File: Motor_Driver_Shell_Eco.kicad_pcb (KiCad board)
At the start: 6 copper layers, 119.6 x 167.9 mm, 214 parts, among them J1 I2C EKRAN, J11 USB_C_Receptacle, J12 Conn_01x02, J13 OUTSIDE LED, J2 HALL INPUT, J3 Conn_01x02, J4 Conn_01x02, J5 Conn_01x04, J6 Conn_01x06, J7 Conn_01x02, J8 Conn_01x03, J9 Conn_01x03, Q1 BC817, Q14 IAUS300N08S5N0, Q15 IAUS300N08S5N0, Q16 IAUS300N08S5N0, Q17 IAUS300N08S5N0, Q18 IAUS300N08S5N0, Q19 IAUS300N08S5N0, Q2 BC817, Q20 IAUS300N08S5N0, Q21 IAUS300N08S5N0, Q6 IAUS300N08S5N0, Q7 IAUS300N08S5N0, Q8 IAUS300N08S5N0, Q9 IAUS300N08S5N0, SW1 SW_Push, SW2 SW_Push, U1 STM32G474VETx, U10 IRS21867S, U11 INA241A2, U12 TMP101, U13 INA241A2, U2 LM5017MR, U3 AP2204K-5.0, U4 XC6206 - 3V3, U5 INA241A2, U6 IRS21867S, U8 TJA1051T, U9 IRS21867S, Y1 8MHz

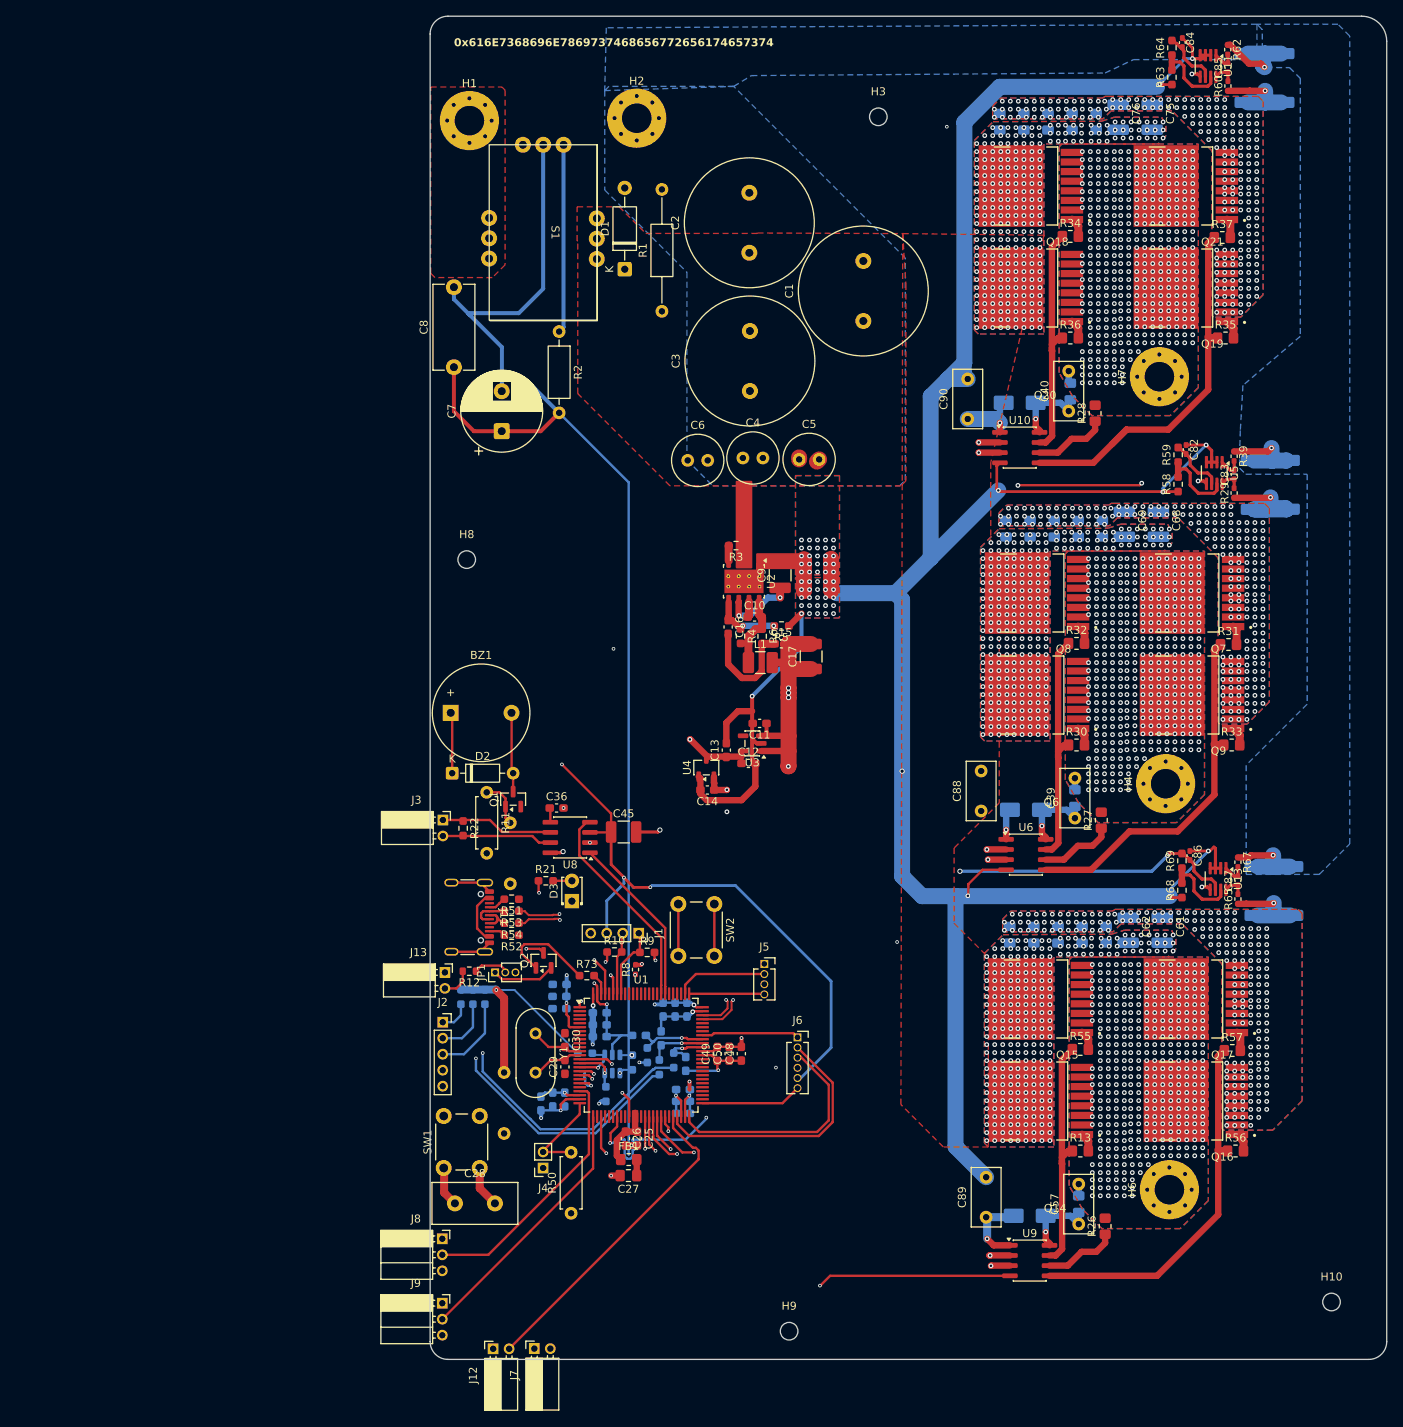
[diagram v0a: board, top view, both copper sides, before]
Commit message: rev3
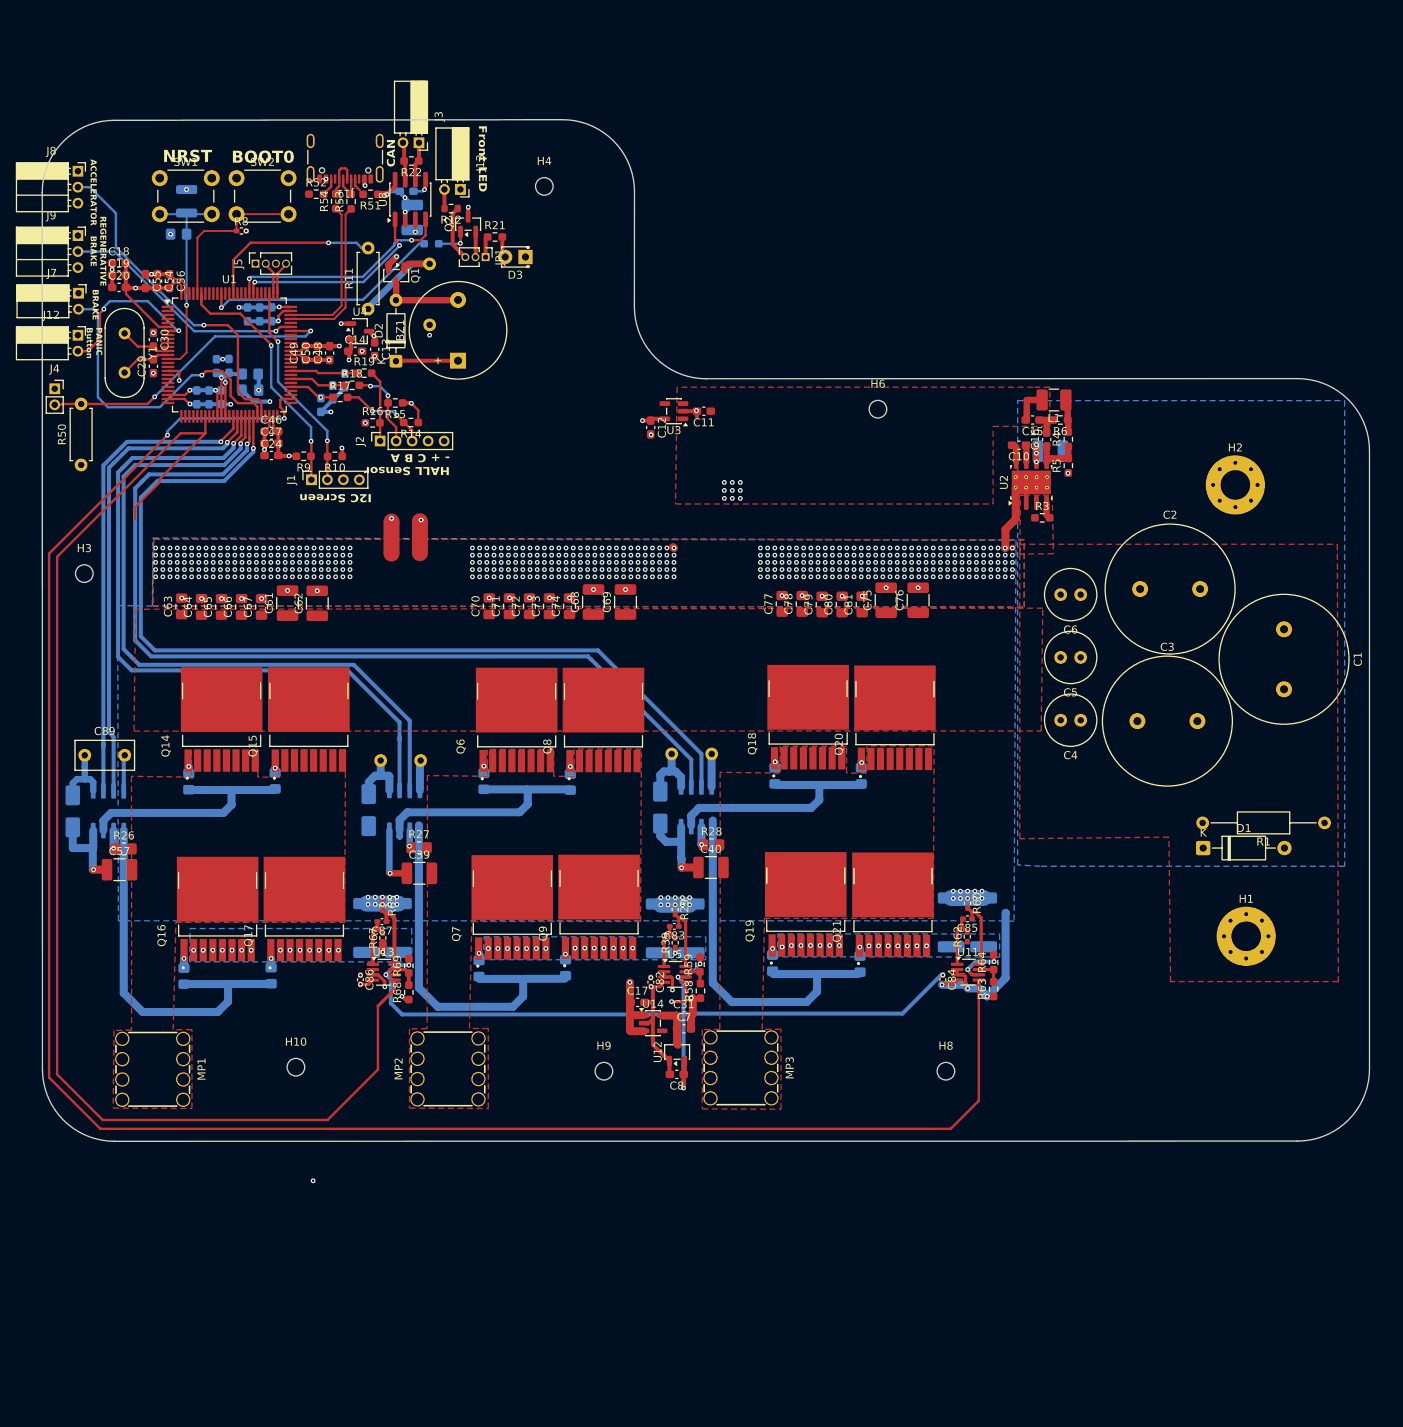
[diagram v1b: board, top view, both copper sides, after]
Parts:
- removed C58, C59, C60: 100uf, Capacitor_SMD:C_0805_2012Metric_Pad1.18x1.45mm_HandSolder
- removed H7: PHASE_C, MountingHole:MountingHole_3.7mm_Pad_Via
- removed J6: Conn_01x06, Connector_PinSocket_1.27mm:PinSocket_1x06_P1.27mm_Vertical
- removed R2: 1K, Resistor_THT:R_Axial_DIN0207_L6.3mm_D2.5mm_P10.16mm_Horizontal
- removed R23: 100, Resistor_SMD:R_0603_1608Metric_Pad0.98x0.95mm_HandSolder
- removed R24, R25: 4.7K, Resistor_SMD:R_0603_1608Metric_Pad0.98x0.95mm_HandSolder
- removed S1: LES50-NP, LES-50NP:LES50NP
- added C31: 2.2uF, Capacitor_SMD:C_0603_1608Metric_Pad1.08x0.95mm_HandSolder, F.Cu at (121.7, 144.6)
- added G***: LOGO, LOGO, B.Cu at (173.7, 134.1)
- added MP1: Phase_A, WP-BUTR:WP-BUTR_7460307, F.Cu at (55.4, 151.3)
- added MP2: Phase_B, WP-BUTR:WP-BUTR_7460307, F.Cu at (92.3, 151.2)
- added MP3: Phase_A, WP-BUTR:WP-BUTR_7460307, F.Cu at (128.9, 151.1)
- added U14: AP2204K-5.0, Package_TO_SOT_SMD:SOT-23-5, F.Cu at (117.9, 145.5)
- C17: value 47uF -> 1uF; footprint Capacitor_SMD:C_1210_3225Metric_Pad1.33x2.70mm_HandSolder -> Capacitor_SMD:C_0603_1608Metric_Pad1.08x0.95mm_HandSolder
- C18, C19, C20, C24, C46, C47, C54, C55, C56, C61, C62, C63, C64, C65, C66, C67, C68, C69, C70, C71, C72, C73, C74, C75, C76, C77, C78, C79, C80, C81, NT2, NT7, R14, R15, R16, R17, R18, R19: moved to F.Cu
- C25, C26, C27, C36, C45, C88, C9, C90, FB1, R13, R30, R31, R32, R33, R34, R35, R36, R37, R55, R56, R57, R73, U10, U6, U9: moved to B.Cu
- C28: footprint Capacitor_THT:C_Disc_D10.5mm_W5.0mm_P5.00mm -> Resistor_SMD:R_0805_2012Metric_Pad1.20x1.40mm_HandSolder; moved to B.Cu
- C39, C40, C57: footprint Capacitor_THT:C_Rect_L7.2mm_W3.5mm_P5.00mm_FKS2_FKP2_MKS2_MKP2 -> Capacitor_SMD:C_1210_3225Metric_Pad1.33x2.70mm_HandSolder
- C7: value 470uF/25V -> 1uF; footprint Capacitor_THT:CP_Radial_D10.0mm_P5.00mm -> Capacitor_SMD:C_0603_1608Metric_Pad1.08x0.95mm_HandSolder
- C8: value 100nF -> 2.2uF; footprint Capacitor_THT:C_Disc_D10.5mm_W5.0mm_P10.00mm -> Capacitor_SMD:C_0603_1608Metric_Pad1.08x0.95mm_HandSolder
- H4: value PHASE_B -> MountingHole; footprint MountingHole:MountingHole_3.7mm_Pad_Via -> MountingHole:MountingHole_2.2mm_M2
- H6: value PHASE_A -> MountingHole; footprint MountingHole:MountingHole_3.7mm_Pad_Via -> MountingHole:MountingHole_2.2mm_M2
- R7: footprint Resistor_THT:R_Axial_DIN0207_L6.3mm_D2.5mm_P7.62mm_Horizontal -> Resistor_SMD:R_1210_3225Metric
- U12: value TMP101 -> XC6206 - 3V3; footprint Package_TO_SOT_SMD:SOT-23-6 -> Package_TO_SOT_SMD:SOT-23-3; moved to F.Cu
- moved J7 143.7 mm to (46.1, 54.2), turned to 0 degrees
- moved J8 141.0 mm to (46.0, 39.0)
- moved J9 141.0 mm to (46.0, 47.0)
- moved H1 140.8 mm to (192.0, 134.6)
- moved J12 136.9 mm to (46.0, 59.5), turned to 0 degrees
- moved R56 133.2 mm to (59.3, 139.6), turned to 90 degrees
- moved H10 132.7 mm to (73.2, 151.0)
- moved R26 131.4 mm to (51.8, 123.7), turned to 0 degrees
- moved D7 129.9 mm to (45.4, 119.0), turned to 90 degrees
- moved SW1 128.7 mm to (56.2, 39.9), turned to 0 degrees
- moved U9 128.1 mm to (49.8, 118.9), turned to -90 degrees
- moved C57 127.8 mm to (51.2, 126.3), turned to 0 degrees
- moved C89 126.6 mm to (46.9, 112.0), turned to 0 degrees
- moved C28 126.0 mm to (58.6, 46.9)
- moved Q16 124.7 mm to (63.5, 131.4), turned to 90 degrees
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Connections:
- C11 pad 2: GND -> -VDC
- C12 pad 2: GND -> -VDC
- C17 pad 2: +12V -> -VDC
- C7 pad 1: CSense_OUT_LES -> +5VD
- C7 pad 2: GND -> -VDC
- C8 pad 1: CSense_OUT_LES -> +3V3F
- C8 pad 2: GND -> -VDC
- C82 pad 1: +3V3 -> +3V3F
- C82 pad 2: GND -> -VDC
- C84 pad 1: +3V3 -> +3V3F
- C84 pad 2: GND -> -VDC
- C86 pad 1: +3V3 -> +3V3F
- C86 pad 2: GND -> -VDC
- C88 pad 2: GND -> -VDC
- C89 pad 2: GND -> -VDC
- C90 pad 2: GND -> -VDC
- H1 pad 1: Net-(H1-Pad1) -> +VDC
- Q16 pad 2: -VDC -> Net-(Q16-Pad2)
- Q16 pad 3: -VDC -> Net-(Q16-Pad2)
- Q16 pad 4: -VDC -> Net-(Q16-Pad2)
- Q16 pad 5: -VDC -> Net-(Q16-Pad2)
- Q16 pad 6: -VDC -> Net-(Q16-Pad2)
- Q16 pad 7: -VDC -> Net-(Q16-Pad2)
- Q16 pad 8: -VDC -> Net-(Q16-Pad2)
- Q17 pad 2: -VDC -> Net-(Q16-Pad2)
- Q17 pad 3: -VDC -> Net-(Q16-Pad2)
- Q17 pad 4: -VDC -> Net-(Q16-Pad2)
- Q17 pad 5: -VDC -> Net-(Q16-Pad2)
- Q17 pad 6: -VDC -> Net-(Q16-Pad2)
- Q17 pad 7: -VDC -> Net-(Q16-Pad2)
- Q17 pad 8: -VDC -> Net-(Q16-Pad2)
- Q19 pad 2: -VDC -> Net-(Q19-Pad2)
- Q19 pad 3: -VDC -> Net-(Q19-Pad2)
- Q19 pad 4: -VDC -> Net-(Q19-Pad2)
- Q19 pad 5: -VDC -> Net-(Q19-Pad2)
- Q19 pad 6: -VDC -> Net-(Q19-Pad2)
- Q19 pad 7: -VDC -> Net-(Q19-Pad2)
- Q19 pad 8: -VDC -> Net-(Q19-Pad2)
- Q2 pad 2: Net-(JP1-A) -> Net-(JP1-C)
- Q21 pad 2: -VDC -> Net-(Q19-Pad2)
- Q21 pad 3: -VDC -> Net-(Q19-Pad2)
- Q21 pad 4: -VDC -> Net-(Q19-Pad2)
- Q21 pad 5: -VDC -> Net-(Q19-Pad2)
- Q21 pad 6: -VDC -> Net-(Q19-Pad2)
- Q21 pad 7: -VDC -> Net-(Q19-Pad2)
- Q21 pad 8: -VDC -> Net-(Q19-Pad2)
- Q7 pad 2: -VDC -> Net-(Q7-Pad2)
- Q7 pad 3: -VDC -> Net-(Q7-Pad2)
- Q7 pad 4: -VDC -> Net-(Q7-Pad2)
- Q7 pad 5: -VDC -> Net-(Q7-Pad2)
- Q7 pad 6: -VDC -> Net-(Q7-Pad2)
- Q7 pad 7: -VDC -> Net-(Q7-Pad2)
- Q7 pad 8: -VDC -> Net-(Q7-Pad2)
- Q9 pad 2: -VDC -> Net-(Q7-Pad2)
- Q9 pad 3: -VDC -> Net-(Q7-Pad2)
- Q9 pad 4: -VDC -> Net-(Q7-Pad2)
- Q9 pad 5: -VDC -> Net-(Q7-Pad2)
- Q9 pad 6: -VDC -> Net-(Q7-Pad2)
- Q9 pad 7: -VDC -> Net-(Q7-Pad2)
- Q9 pad 8: -VDC -> Net-(Q7-Pad2)
- R12 pad 1: Net-(JP1-C) -> Net-(JP1-B)
- R21 pad 1: Net-(JP1-B) -> Net-(JP1-A)
- R38 pad 2: -VDC -> Net-(Q7-Pad2)
- R39 pad 1: -VDC -> Net-(Q7-Pad2)
- R5 pad 1: GND -> -VDC
- R58 pad 1: GND -> -VDC
- R59 pad 2: +3V3 -> +3V3F
- R61 pad 2: -VDC -> Net-(Q19-Pad2)
- R62 pad 1: -VDC -> Net-(Q19-Pad2)
- R63 pad 1: GND -> -VDC
- R64 pad 2: +3V3 -> +3V3F
- R66 pad 1: -VDC -> Net-(Q16-Pad2)
- R67 pad 1: -VDC -> Net-(Q16-Pad2)
- R68 pad 1: GND -> -VDC
- R69 pad 2: +3V3 -> +3V3F
- R70 pad 2: -VDC -> Net-(Q7-Pad2)
- R71 pad 2: -VDC -> Net-(Q16-Pad2)
- R72 pad 2: -VDC -> Net-(Q19-Pad2)
- U1 pad 1: BRAKE -> unconnected-(U1-PE2-Pad1)
- U1 pad 15: TMP_SDA -> unconnected-(U1-PC0-Pad15)
- U1 pad 16: TMP_SCL -> unconnected-(U1-PC1-Pad16)
- U1 pad 18: TMP_ALERT -> unconnected-(U1-PC3-Pad18)
- U1 pad 20: CSense_OUT_LES -> unconnected-(U1-PA0-Pad20)
- U1 pad 21: B_VOL_CHECK -> unconnected-(U1-PA1-Pad21)
- U1 pad 22: ACCEL -> unconnected-(U1-PA2-Pad22)
- U1 pad 25: TEMP_SENSOR -> unconnected-(U1-PA3-Pad25)
- U1 pad 26: REGEN -> unconnected-(U1-PA4-Pad26)
- U1 pad 28: Current Sense_A -> unconnected-(U1-PA6-Pad28)
- U1 pad 32: Current_Sense_C -> Current Sense_A
- U1 pad 39: /FET/LS_MOS_A -> /FET/HS_MOS_A
- U1 pad 40: /FET/HS_MOS_A -> /FET/LS_MOS_A
- U1 pad 45: unconnected-(U1-PE14-Pad45) -> BRAKE
- U1 pad 46: PANIC STOP -> ACCEL
- U1 pad 47: BT_TX -> unconnected-(U1-PB10-Pad47)
- U1 pad 50: BT_RX -> unconnected-(U1-PB11-Pad50)
- U1 pad 51: BT_KEY -> unconnected-(U1-PB12-Pad51)
- U1 pad 52: unconnected-(U1-PB13-Pad52) -> Current_Sense_C
- U1 pad 55: unconnected-(U1-PD8-Pad55) -> HALL_C
- U1 pad 57: unconnected-(U1-PD10-Pad57) -> HALL_B
- U1 pad 59: unconnected-(U1-PD12-Pad59) -> HALL_A
- U1 pad 65: HALL_A -> unconnected-(U1-PC6-Pad65)
- U1 pad 66: HALL_B -> unconnected-(U1-PC7-Pad66)
- U1 pad 67: HALL_C -> unconnected-(U1-PC8-Pad67)
- U1 pad 68: BT_STATE -> unconnected-(U1-PC9-Pad68)
- U1 pad 69: unconnected-(U1-PA8-Pad69) -> TEMP_SENSOR
- U1 pad 7: unconnected-(U1-PC13-Pad7) -> PANIC STOP
- U1 pad 70: unconnected-(U1-PA9-Pad70) -> REGEN
- U1 pad 78: unconnected-(U1-PA15-Pad78) -> /MCU/I2C_SDA
- U1 pad 87: unconnected-(U1-PD5-Pad87) -> BUZZER
- U1 pad 90: unconnected-(U1-PB3-Pad90) -> STATUS_LED
- U1 pad 93: /MCU/I2C_SCL -> unconnected-(U1-PB6-Pad93)
- U1 pad 94: /MCU/I2C_SDA -> unconnected-(U1-PB7-Pad94)
- U1 pad 95: /MCU/BOOT0 -> /MCU/I2C_SCL
- U1 pad 96: unconnected-(U1-PB9-Pad96) -> /MCU/BOOT0
- U1 pad 97: BUZZER -> unconnected-(U1-PE0-Pad97)
- U1 pad 98: STATUS_LED -> unconnected-(U1-PE1-Pad98)
- U10 pad 4: GND -> -VDC
- U11 pad 2: GND -> -VDC
- U11 pad 3: GND -> -VDC
- U11 pad 4: GND -> -VDC
- U11 pad 6: +3V3 -> +3V3F
- U12 pad 1: TMP_SCL -> -VDC
- U12 pad 2: GND -> +3V3F
- U12 pad 3: TMP_ALERT -> +5VD
- U13 pad 2: GND -> -VDC
- U13 pad 3: GND -> -VDC
- U13 pad 4: GND -> -VDC
- U13 pad 6: +3V3 -> +3V3F
- U3 pad 2: GND -> -VDC
- U5 pad 2: GND -> -VDC
- U5 pad 3: GND -> -VDC
- U5 pad 4: GND -> -VDC
- U5 pad 6: +3V3 -> +3V3F
- U6 pad 4: GND -> -VDC
- U9 pad 4: GND -> unconnected-(U9-COM-Pad4)
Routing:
- net GND: track 585.4 -> 60.9 mm, vias 52 -> 24
- net +5V: track 258.3 -> 23.7 mm, vias 5 -> 6
- net +3V3: track 141.4 -> 10.6 mm, vias 15 -> 11
- net CSense_OUT_LES: track 125.4 -> 0.00 mm, vias 1 -> 0
- net +3V3F: track 0.00 -> 121.2 mm, vias 0 -> 10
- net -VDC: track 76.8 -> 154.9 mm, vias 673 -> 528
- net Current Sense_A: track 103.0 -> 163.3 mm, vias 3 -> 0
- net Current_Sense_C: track 200.7 -> 241.5 mm, vias 4 -> 2
- net Net-(J2-Pin_1): track 44.9 -> 8.93 mm, vias 1 -> 0
- net Net-(J2-Pin_3): track 46.2 -> 11.2 mm, vias 1 -> 2
- net Net-(J2-Pin_2): track 43.9 -> 10.3 mm, vias 1 -> 2
- net BT_TX: track 32.8 -> 0.00 mm
- net Current Sense_B: track 163.4 -> 192.8 mm, vias 4 -> 2
- net BT_RX: track 29.1 -> 0.00 mm
- net STATUS_LED: track 2.64 -> 30.4 mm, vias 0 -> 1
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- added copper zone on F.Cu, net +12V
- added copper zone on In2.Cu, net +3V3
- added copper zone on In2.Cu, net +5V
- added copper zone on B.Cu, net Net-(Q16-Pad2)
- added copper zone on B.Cu, net Net-(Q19-Pad2)
- added copper zone on B.Cu, net Net-(Q7-Pad2)
- removed copper zone on In3.Cu, net +3V3
- removed copper zone on B.Cu, net +VDC
- removed copper zone on In1.Cu, net +VDC
- removed copper zone on In2.Cu, net +VDC
- removed copper zone on In4.Cu, net +VDC
- removed copper zone on In1.Cu, net -VDC
- removed copper zone on In3.Cu, net -VDC
- removed copper zone on In4.Cu, net -VDC
- removed copper zone on B.Cu, net /FET/Phase_A_FET/PHASE_A
- removed copper zone on In2.Cu, net /FET/Phase_A_FET/PHASE_A
- removed copper zone on In3.Cu, net /FET/Phase_A_FET/PHASE_A
- removed copper zone on In4.Cu, net /FET/Phase_A_FET/PHASE_A
- removed copper zone on B.Cu, net /FET/Phase_B_FET/PHASE_B
- removed copper zone on In2.Cu, net /FET/Phase_B_FET/PHASE_B
- removed copper zone on In3.Cu, net /FET/Phase_B_FET/PHASE_B
- removed copper zone on In4.Cu, net /FET/Phase_B_FET/PHASE_B
- removed copper zone on B.Cu, net /FET/Phase_C_FET/PHASE_C
- removed copper zone on In2.Cu, net /FET/Phase_C_FET/PHASE_C
- removed copper zone on In3.Cu, net /FET/Phase_C_FET/PHASE_C
- removed copper zone on In4.Cu, net /FET/Phase_C_FET/PHASE_C
- removed copper zone on B.Cu, net GND
- removed copper zone on F.Cu, net GND
- removed copper zone on In2.Cu, net GND
- removed copper zone on In3.Cu, net GND
- removed copper zone on In4.Cu, net GND
- removed copper zone on F.Cu, net Net-(H1-Pad1)
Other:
- board size 119.6 x 167.9 mm -> 165.9 x 127.7 mm
- copper layers 6 -> 4
- board text added: "ACCELERATOR"
- board text added: "BOOT0"
- board text added: "BRAKE"
- board text added: "CAN"
- board text added: "Front LED"
- board text added: "HALL Sensor - + C B A"
- board text added: "I2C Screen"
- board text added: "NRST"
- board text added: "PANIC Button"
- board text added: "PEHLI-MD by Yener S. {dblquote}Anshinx{dblquote} Güneş For Pehlivan Team's use @ Shell Eco Marathon rev 0.3"
- board text added: "REGENERATIVE BRAKE"
- board text added: "SEM"
- board text removed: "0x616E7368696E7869737468656772656174657374"
- board text removed: "0x73766D2E62682E676E636B2E692E6D2E6C0A"
- board text removed: "SEM 2026"
